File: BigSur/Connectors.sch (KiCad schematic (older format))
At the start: 36 parts, among them J1 XT30PW-M, J10 XT30PW-M, J11 Conn_01x03, J12 XT30PW-M, J13 Conn_01x04, J14 XT30PW-M, J15 XT30PW-M, J16 XT30PW-M, J2 XT30PW-M, J3 XT30PW-M, J4 XT30PW-M, J5 XT30PW-M, J6 XT30PW-M, J7 XT30PW-M, J8 XT30PW-M, J9 XT30PW-M, U4 SMD46

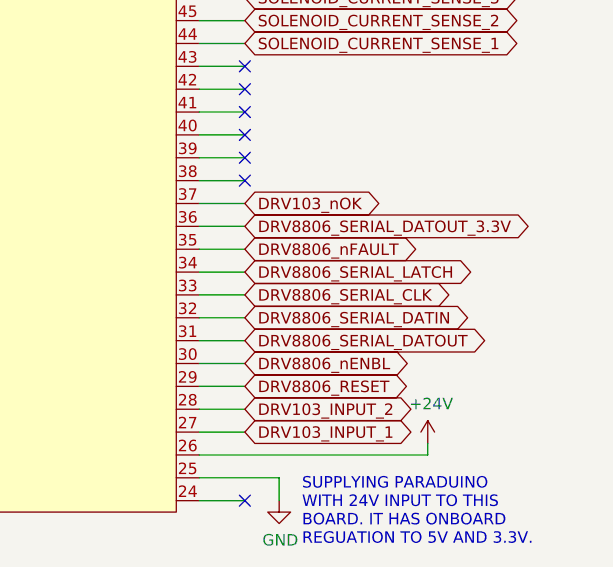
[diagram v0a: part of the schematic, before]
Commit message: Finished another layout pass.
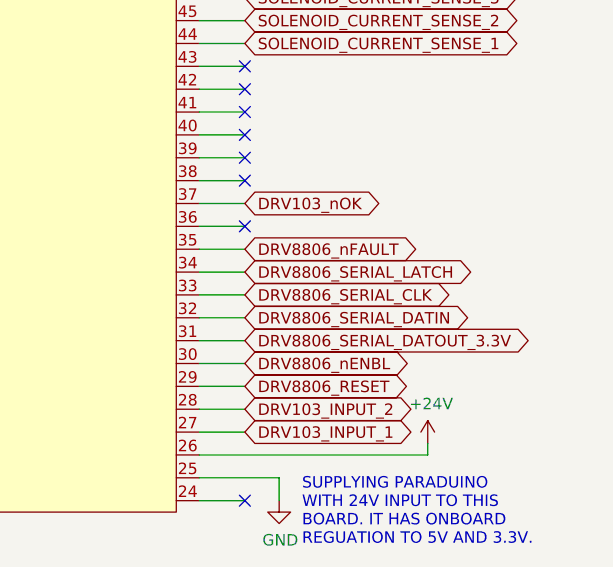
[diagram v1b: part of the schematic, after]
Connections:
- net DRV8806_SERIAL_DATOUT is gone; now on net DRV8806_SERIAL_DATOUT_3.3V: U4.31
- net DRV8806_SERIAL_DATOUT_3.3V: no longer U4.36
- no-connect marks 10 -> 11
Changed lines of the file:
@@
 Wire Wire Line
 	9650 3200 9450 3200
-Text GLabel 9650 3200 2    50   BiDi ~ 0
-DRV8806_SERIAL_DATOUT
 Wire Wire Line
 	9650 3300 9450 3300
@@
 Text GLabel 9650 2800 2    50   BiDi ~ 0
 DRV8806_nFAULT
-Text GLabel 9650 2700 2    50   BiDi ~ 0
+Text GLabel 9650 3200 2    50   BiDi ~ 0
 DRV8806_SERIAL_DATOUT_3.3V
 Text GLabel 9650 2600 2    50   BiDi ~ 0
@@
 	1    0    0    -1
 $EndComp
+NoConn ~ 9650 2700
 $EndSCHEMATC
